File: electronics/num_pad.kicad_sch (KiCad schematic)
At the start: 37 parts, among them J10 Conn_01x05_Male, J9 Conn_01x05_Female, SW69 SW_SPST, SW70 SW_SPST, SW71 SW_SPST, SW72 SW_SPST, SW73 SW_SPST, SW74 SW_SPST, SW75 SW_SPST, SW76 SW_SPST, SW77 SW_SPST, SW78 SW_SPST, SW79 SW_SPST, SW80 SW_SPST, SW81 SW_SPST, SW82 SW_SPST, SW83 SW_SPST, SW84 SW_SPST, SW85 SW_SPST, U5 PCA9675PW

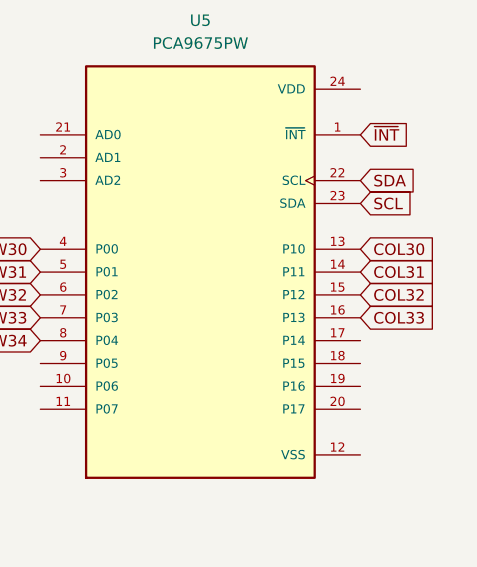
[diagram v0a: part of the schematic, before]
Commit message: finish matrix
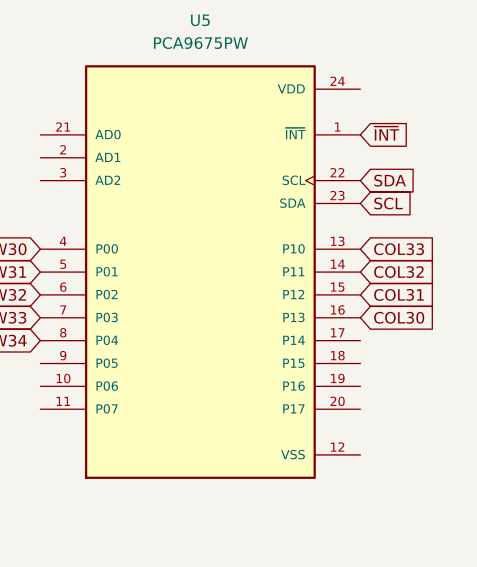
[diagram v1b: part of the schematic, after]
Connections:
- net COL30: now also U5.16 (P13); no longer U5.13 (P10)
- net COL31: now also U5.15 (P12); no longer U5.14 (P11)
- net COL32: now also U5.14 (P11); no longer U5.15 (P12)
- net COL33: now also U5.13 (P10); no longer U5.16 (P13)
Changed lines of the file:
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@@
     (stroke (width 0) (type default) (color 0 0 0 0))
   )
+  (global_label "COL30" (shape input) (at 237.49 66.04 0) (fields_autoplaced)
+    (effects (font (size 1.27 1.27)) (justify left))
+    (property "Intersheet References" "${INTERSHEET_REFS}" (id 0) (at 245.9507 65.9606 0)
+      (effects (font (size 1.27 1.27)) (justify left) hide)
+    )
+  )
   (global_label "ROW30" (shape input) (at 55.88 101.6 180) (fields_autoplaced)
     (effects (font (size 1.27 1.27)) (justify right))
@@
     )
   )
-  (global_label "COL32" (shape input) (at 237.49 63.5 0) (fields_autoplaced)
-    (effects (font (size 1.27 1.27)) (justify left))
-    (property "Intersheet References" "${INTERSHEET_REFS}" (id 0) (at 245.9507 63.5794 0)
-      (effects (font (size 1.27 1.27)) (justify left) hide)
-    )
-  )
   (global_label "ROW34" (shape input) (at 96.52 165.1 180) (fields_autoplaced)
     (effects (font (size 1.27 1.27)) (justify right))
@@
     )
   )
+  (global_label "COL33" (shape input) (at 237.49 58.42 0) (fields_autoplaced)
+    (effects (font (size 1.27 1.27)) (justify left))
+    (property "Intersheet References" "${INTERSHEET_REFS}" (id 0) (at 245.9507 58.3406 0)
+      (effects (font (size 1.27 1.27)) (justify left) hide)
+    )
+  )
   (global_label "ROW30" (shape input) (at 96.52 101.6 180) (fields_autoplaced)
     (effects (font (size 1.27 1.27)) (justify right))
@@
     )
   )
-  (global_label "COL31" (shape input) (at 237.49 60.96 0) (fields_autoplaced)
-    (effects (font (size 1.27 1.27)) (justify left))
-    (property "Intersheet References" "${INTERSHEET_REFS}" (id 0) (at 245.9507 61.0394 0)
-      (effects (font (size 1.27 1.27)) (justify left) hide)
-    )
-  )
   (global_label "COL33" (shape input) (at 127 82.55 180) (fields_autoplaced)
     (effects (font (size 1.27 1.27)) (justify right))
@@
     )
   )
-  (global_label "COL30" (shape input) (at 237.49 58.42 0) (fields_autoplaced)
-    (effects (font (size 1.27 1.27)) (justify left))
-    (property "Intersheet References" "${INTERSHEET_REFS}" (id 0) (at 245.9507 58.4994 0)
-      (effects (font (size 1.27 1.27)) (justify left) hide)
-    )
-  )
   (global_label "~{INT}" (shape input) (at 237.49 45.72 0) (fields_autoplaced)
     (effects (font (size 1.27 1.27)) (justify left))
@@
     )
   )
-  (global_label "COL33" (shape input) (at 237.49 66.04 0) (fields_autoplaced)
-    (effects (font (size 1.27 1.27)) (justify left))
-    (property "Intersheet References" "${INTERSHEET_REFS}" (id 0) (at 245.9507 66.1194 0)
-      (effects (font (size 1.27 1.27)) (justify left) hide)
-    )
-  )
   (global_label "ROW33" (shape input) (at 76.2 149.86 180) (fields_autoplaced)
     (effects (font (size 1.27 1.27)) (justify right))
@@
     )
   )
+  (global_label "COL31" (shape input) (at 237.49 63.5 0) (fields_autoplaced)
+    (effects (font (size 1.27 1.27)) (justify left))
+    (property "Intersheet References" "${INTERSHEET_REFS}" (id 0) (at 245.9507 63.4206 0)
+      (effects (font (size 1.27 1.27)) (justify left) hide)
+    )
+  )
   (global_label "ROW33" (shape input) (at 201.93 66.04 180) (fields_autoplaced)
     (effects (font (size 1.27 1.27)) (justify right))
@@
       (effects (font (size 1.27 1.27)) (justify left) hide)
     )
+  )
+  (global_label "COL32" (shape input) (at 237.49 60.96 0) (fields_autoplaced)
+    (effects (font (size 1.27 1.27)) (justify left))
+    (property "Intersheet References" "${INTERSHEET_REFS}" (id 0) (at 245.9507 60.8806 0)
+      (effects (font (size 1.27 1.27)) (justify left) hide)
+    )
